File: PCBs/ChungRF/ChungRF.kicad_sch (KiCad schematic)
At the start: 11 parts, among them J1 JST-SM04B-SRSS, J2 Conn_Coaxial, U1 KB2040, U2 E22-900M30S

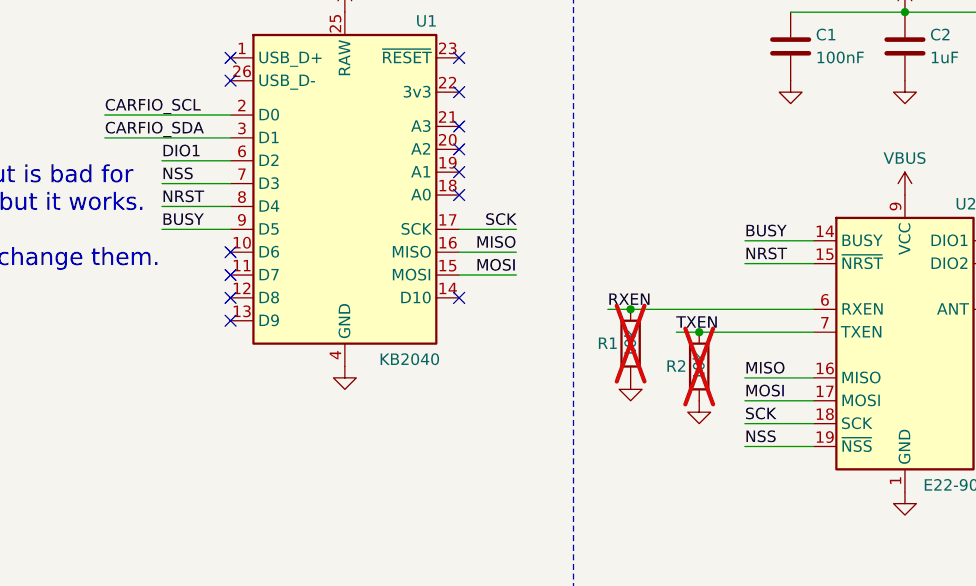
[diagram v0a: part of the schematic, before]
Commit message: Clean Tracks, add Gerber files
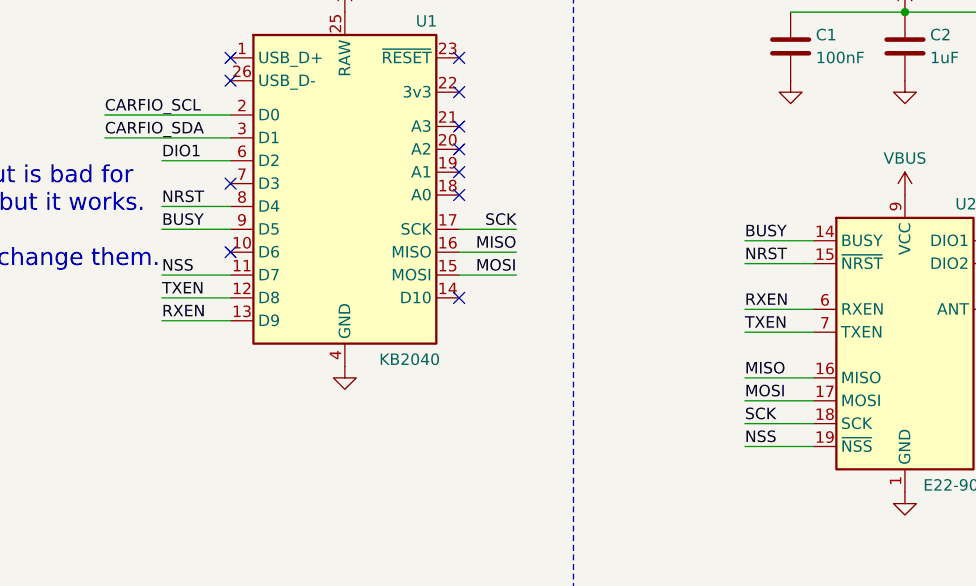
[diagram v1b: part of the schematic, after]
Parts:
- removed R1, R2: 10k, Capacitor_SMD:C_0603_1608Metric, symbol Device:R
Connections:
- net NSS: now also U1.11 (D7); no longer U1.7 (D3)
- net RXEN: now also U1.13 (D9)
- net TXEN: now also U1.12 (D8)
- no-connect marks 14 -> 12
